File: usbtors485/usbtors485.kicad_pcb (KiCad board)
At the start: 2 copper layers, 8 parts, among them IC9 THVD1426DRLR

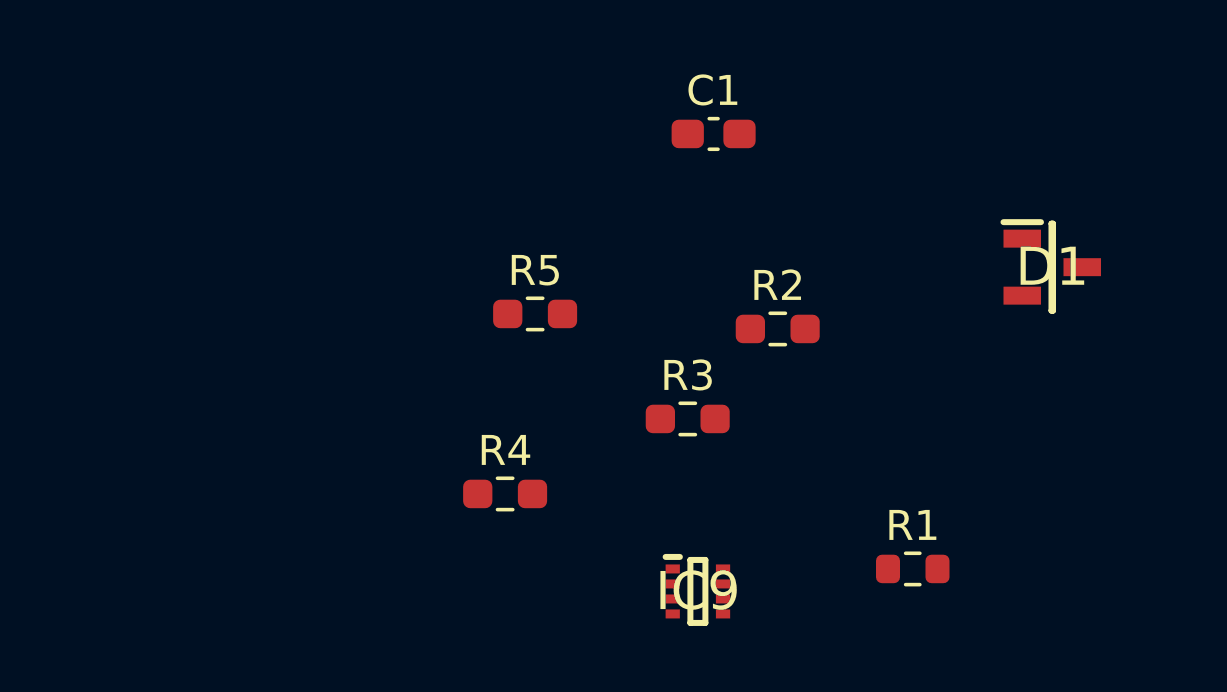
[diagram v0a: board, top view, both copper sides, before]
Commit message: update design
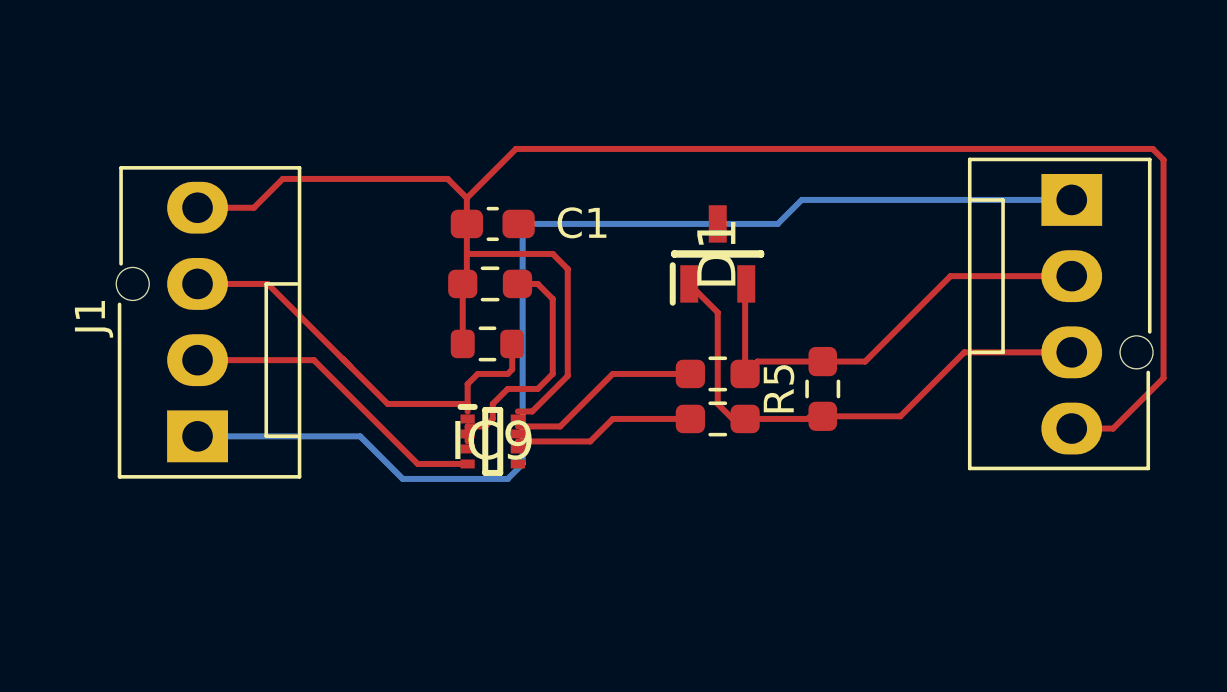
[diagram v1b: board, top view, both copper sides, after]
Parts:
- added J1: ~, Connector:FanPinHeader_1x04_P2.54mm_Vertical, F.Cu at (118.2, 85.1)
- added J2: Conn_01x04_Socket, Connector:FanPinHeader_1x04_P2.54mm_Vertical, F.Cu at (147.3, 77.2)
- moved R1 16.0 mm to (127.8, 82.0)
- moved D1 11.2 mm to (135.5, 79.0), turned to 90 degrees
- moved R5 9.91 mm to (139.0, 83.5), turned to 90 degrees
- moved R2 9.70 mm to (127.9, 80.0)
- moved IC9 8.47 mm to (128.0, 85.2)
- moved C1 7.95 mm to (128.0, 78.0)
- moved R4 7.52 mm to (135.5, 84.5)
- moved R3 1.80 mm to (135.5, 83.0)
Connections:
- IC9 pad 4: unconnected-(IC9-D-Pad4) -> Net-(IC9-D)
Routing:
- net VDD: track 0.00 -> 58.9 mm
- net GND: track 0.00 -> 38.3 mm
- net Net-(J2-Pin_3): track 0.00 -> 17.3 mm
- net Net-(J2-Pin_2): track 0.00 -> 15.3 mm
- net /UART RX: track 0.00 -> 14.5 mm
- net Net-(IC9-D): track 0.00 -> 10.4 mm
- net Net-(IC9-~{RE}): track 0.00 -> 8.24 mm
- net Net-(IC9-B): track 0.00 -> 6.47 mm
- net Net-(IC9-A): track 0.00 -> 6.06 mm
